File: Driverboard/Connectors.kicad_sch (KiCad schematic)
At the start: 23 parts, among them IC7 TPS25810RVCT, J1 Motor Driver 2, J10 EN_Input, J11 Z/F_Input, J12 EN_Z/F_MD3, J13 EN_Z/F_MD4, J14 USB_C_Receptacle_USB2.0, J2 Motor Driver 4, J3 Speed_Input, J4 Conn_01x16, J5 EN_Z/F_MD1, J6 EN_Z/F_MD2, J7 Speed_Output, J8 Motor Driver 1, J9 Motor Driver 3, U2 ISL43240IAZ-T, U3 ISL43240IAZ-T

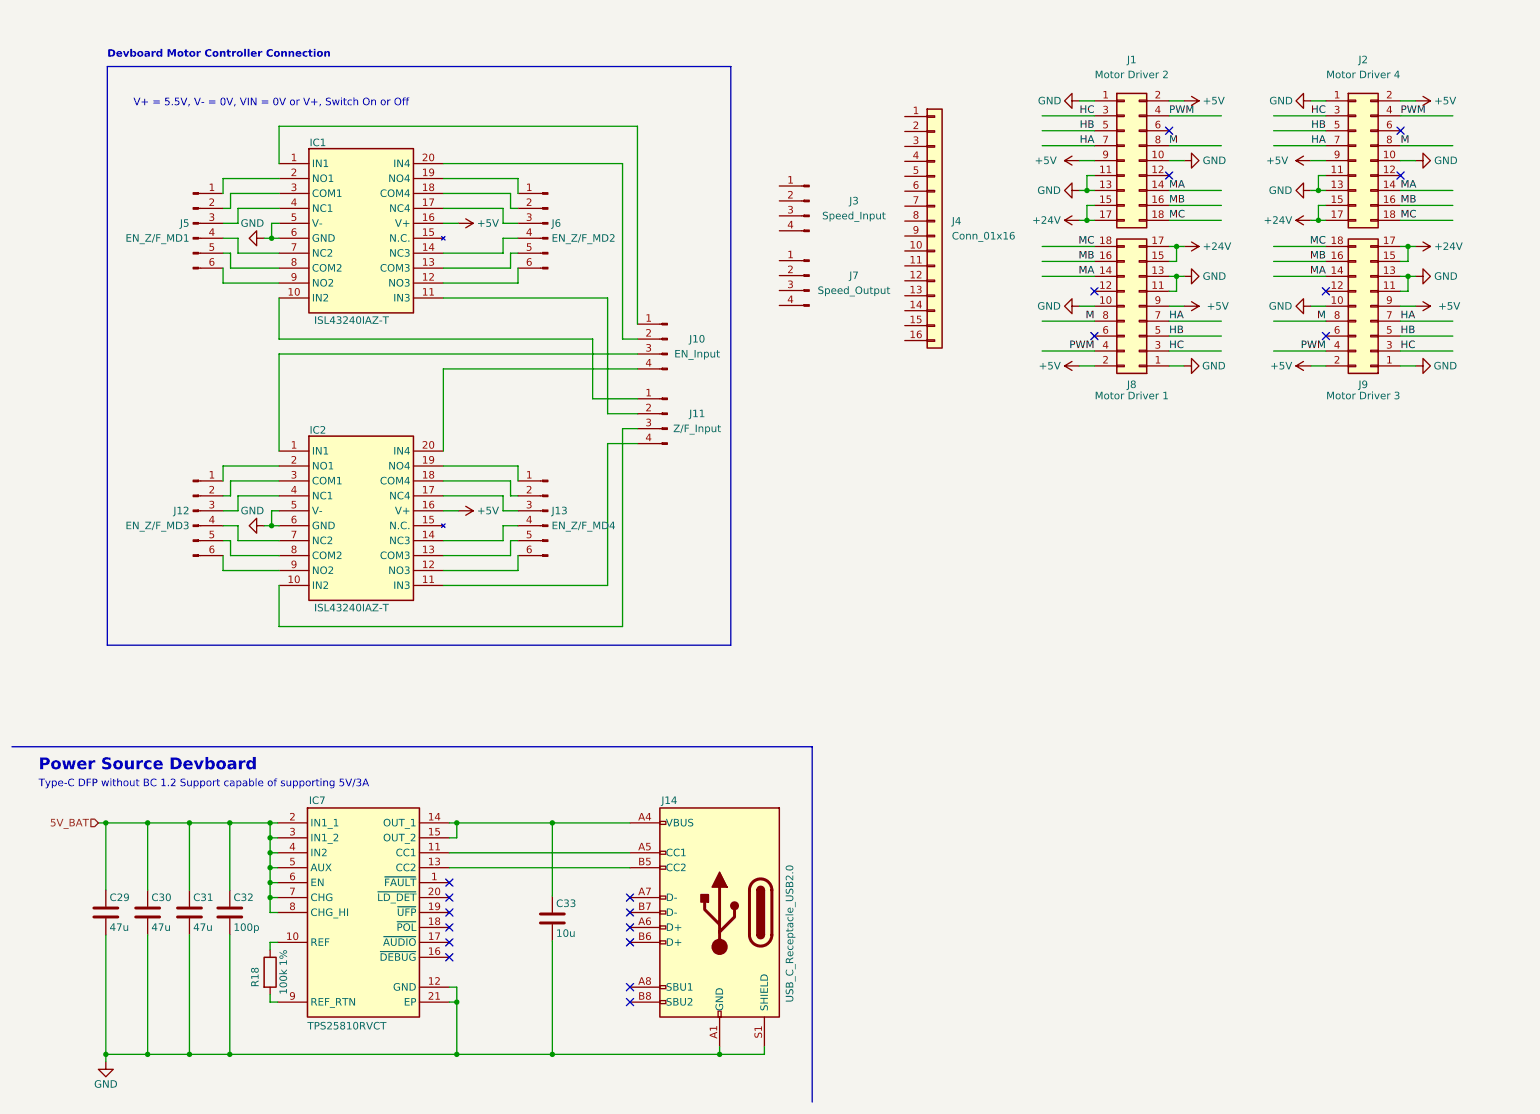
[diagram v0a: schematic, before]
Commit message: WIP
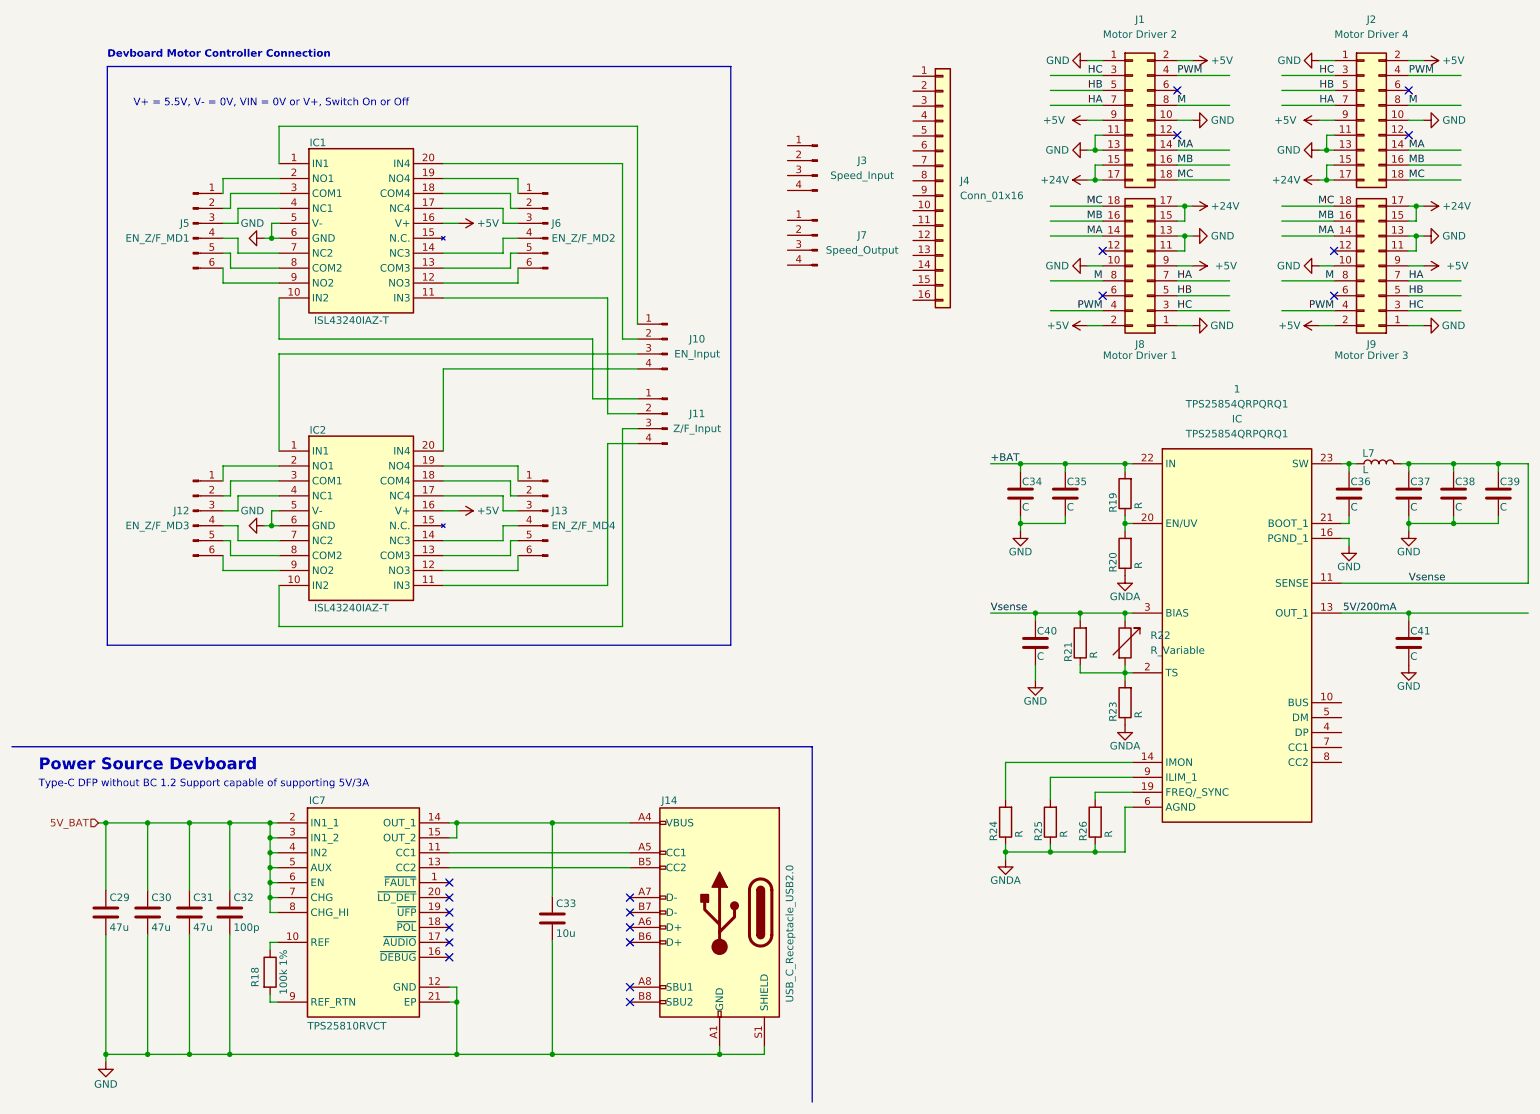
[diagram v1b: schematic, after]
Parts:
- added 1: TPS25854QRPQRQ1, symbol TPS25854QRPQRQ1:TPS25854QRPQRQ1
- added C34, C35, C36, C37, C38, C39, C40, C41: C, symbol Device:C
- added L7: L, symbol Device:L
- added R19, R20, R21, R23, R24, R25, R26: R, symbol Device:R
- added R22: R_Variable, symbol Device:R_Variable
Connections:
- net GND: now also 1.16 (PGND_1), 1.24 (PGND_2), 1.25 (PGND_3), C34.2, C35.2, C37.2, C38.2, C39.2, C40.2, C41.2
- new net: 1.23 (SW), C36.1, L7.1
- new net: 1.21 (BOOT_1), 1.29 (BOOT_2), C36.2
- new net: 1.2 (TS), R21.1, R22.2, R23.2
- new net: 1.20 (EN/UV), R19.1, R20.2
- new net: 1.1 (NC_1), 1.12 (NC_2), 1.26 (NC_3)
- new net: 1.14 (IMON), R24.2
- new net: 1.15 (~{THERM_WARN}), 1.17 (~{POL}), 1.18 (~{FAULT})
- new net: 1.19 (FREQ/_SYNC), R26.2
- new net: 1.27 (ILIM_2), 1.9 (ILIM_1), R25.2
- new net +BAT: 1.22 (IN), C34.1, C35.1, R19.2
- new net 5V/200mA: 1.13 (OUT_1), 1.28 (OUT_2), C41.1
- new net GNDA: 1.6 (AGND), R20.1, R23.1, R24.1, R25.1, R26.1
- new net Vsense: 1.11 (SENSE), 1.3 (BIAS), C37.1, C38.1, C39.1, C40.1, L7.2, R21.2, R22.1
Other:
- moved on the sheet: J1, J2, J3, J4, J7, J8, J9
